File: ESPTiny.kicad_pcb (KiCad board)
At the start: 2 copper layers, 33 x 26.4 mm, 16 parts, among them J1 Conn_01x10_Male, J2 Conn_01x10_Male, J3 Conn_01x04_Male, U1 ESP-01v090, U2 ATtiny84-20PU, U3 MCP1700-3302E_TO92

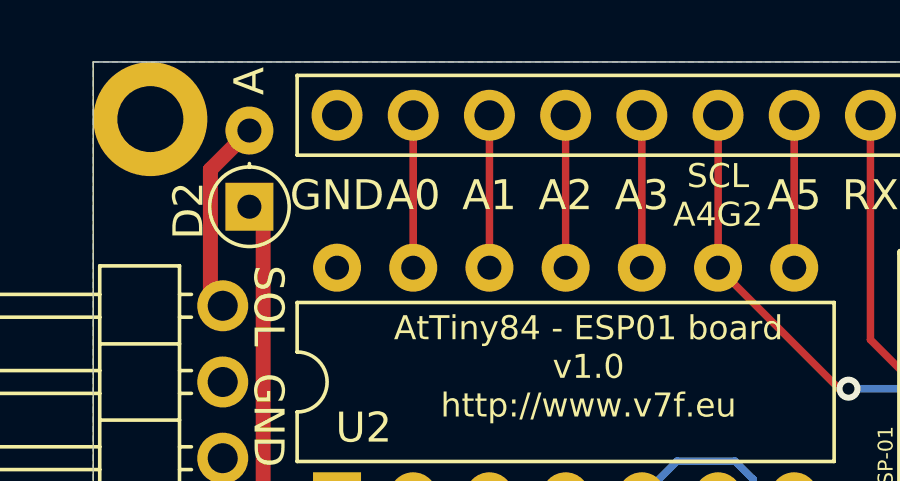
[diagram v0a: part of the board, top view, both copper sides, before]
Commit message: With power divider
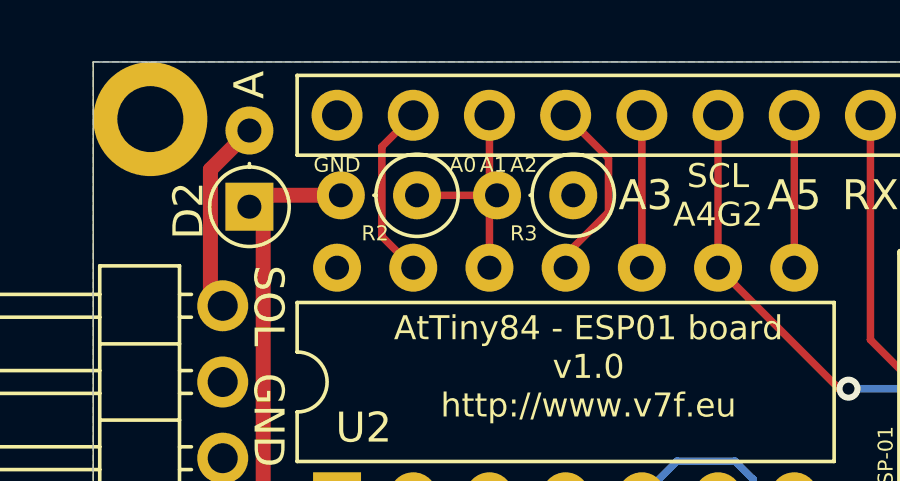
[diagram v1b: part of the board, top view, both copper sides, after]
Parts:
- added R2: 220, Resistor_THT:R_Axial_DIN0207_L6.3mm_D2.5mm_P2.54mm_Vertical, F.Cu at (49.9, 44.8)
- added R3: 220, Resistor_THT:R_Axial_DIN0207_L6.3mm_D2.5mm_P2.54mm_Vertical, F.Cu at (55.1, 44.8)
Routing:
- net +BATT: track 21.2 -> 24.4 mm
- net /A1: track 5.08 -> 7.96 mm
- net /A2: track 5.08 -> 6.26 mm
- net /A0: track 5.08 -> 5.95 mm
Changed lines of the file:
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@@
     (thickness 1.6)
     (drawings 49)
-    (tracks 122)
+    (tracks 133)
     (zones 0)
-    (modules 16)
+    (modules 18)
     (nets 21)
   )
@@
   )
   (layers
-    (0 F.Cu signal hide)
-    (31 B.Cu signal hide)
+    (0 F.Cu signal)
+    (31 B.Cu signal)
     (32 B.Adhes user)
     (33 F.Adhes user)
@@
       (effects (font (size 1 1) (thickness 0.15)))
     )
-    (fp_text user A (at 4.191 0 90) (layer F.SilkS)
+    (fp_text user A (at 4.064 0 90) (layer F.SilkS)
       (effects (font (size 1 1) (thickness 0.15)))
     )
@@
     )
   )
+  (module Resistor_THT:R_Axial_DIN0207_L6.3mm_D2.5mm_P2.54mm_Vertical (layer F.Cu)
+    (at 49.911 44.831 180)
+    (descr "Resistor, Axial_DIN0207 series, Axial, Vertical, pin pitch=2.54mm, 0.25W = 1/4W, length*diameter=6.3*2.5mm^2, http://cdn-reichelt.de/documents/datenblatt/B400/1_4W%23YAG.pdf")
+    (tags "Resistor Axial_DIN0207 series Axial Vertical pin pitch 2.54mm 0.25W = 1/4W length 6.3mm diameter 2.5mm")
+    (fp_text reference R2 (at 1.397 -1.27) (layer F.SilkS)
+      (effects (font (size 0.5 0.5) (thickness 0.125)))
+    )
+    (fp_text value 220 (at 1.27 2.37) (layer F.Fab)
+      (effects (font (size 1 1) (thickness 0.15)))
+    )
+    (fp_line (start 3.59 -1.5) (end -1.5 -1.5) (layer F.CrtYd) (width 0.05))
+    (fp_line (start 3.59 1.5) (end 3.59 -1.5) (layer F.CrtYd) (width 0.05))
+    (fp_line (start -1.5 1.5) (end 3.59 1.5) (layer F.CrtYd) (width 0.05))
+    (fp_line (start -1.5 -1.5) (end -1.5 1.5) (layer F.CrtYd) (width 0.05))
+    (fp_line (start 1.37 0) (end 1.44 0) (layer F.SilkS) (width 0.12))
+    (fp_line (start 0 0) (end 2.54 0) (layer F.Fab) (width 0.1))
+    (fp_circle (center 0 0) (end 1.37 0) (layer F.SilkS) (width 0.12))
+    (fp_circle (center 0 0) (end 1.25 0) (layer F.Fab) (width 0.1))
+    (fp_text user %R (at 1.27 -2.37) (layer F.Fab)
+      (effects (font (size 1 1) (thickness 0.15)))
+    )
+    (pad 1 thru_hole circle (at 0 0 180) (size 1.6 1.6) (drill 0.8) (layers *.Cu *.Mask)
+      (net 19 /A1))
+    (pad 2 thru_hole oval (at 2.54 0 180) (size 1.6 1.6) (drill 0.8) (layers *.Cu *.Mask)
+      (net 5 +BATT))
+    (model ${KISYS3DMOD}/Resistor_THT.3dshapes/R_Axial_DIN0207_L6.3mm_D2.5mm_P2.54mm_Vertical.wrl
+      (at (xyz 0 0 0))
+      (scale (xyz 1 1 1))
+      (rotate (xyz 0 0 0))
+    )
+  )
+  (module Resistor_THT:R_Axial_DIN0207_L6.3mm_D2.5mm_P2.54mm_Vertical (layer F.Cu)
+    (at 55.118 44.831 180)
+    (descr "Resistor, Axial_DIN0207 series, Axial, Vertical, pin pitch=2.54mm, 0.25W = 1/4W, length*diameter=6.3*2.5mm^2, http://cdn-reichelt.de/documents/datenblatt/B400/1_4W%23YAG.pdf")
+    (tags "Resistor Axial_DIN0207 series Axial Vertical pin pitch 2.54mm 0.25W = 1/4W length 6.3mm diameter 2.5mm")
+    (fp_text reference R3 (at 1.651 -1.27) (layer F.SilkS)
+      (effects (font (size 0.5 0.5) (thickness 0.125)))
+    )
+    (fp_text value 220 (at 1.27 2.37) (layer F.Fab)
+      (effects (font (size 1 1) (thickness 0.15)))
+    )
+    (fp_text user %R (at 1.27 -2.37) (layer F.Fab)
+      (effects (font (size 1 1) (thickness 0.15)))
+    )
+    (fp_circle (center 0 0) (end 1.25 0) (layer F.Fab) (width 0.1))
+    (fp_circle (center 0 0) (end 1.37 0) (layer F.SilkS) (width 0.12))
+    (fp_line (start 0 0) (end 2.54 0) (layer F.Fab) (width 0.1))
+    (fp_line (start 1.37 0) (end 1.44 0) (layer F.SilkS) (width 0.12))
+    (fp_line (start -1.5 -1.5) (end -1.5 1.5) (layer F.CrtYd) (width 0.05))
+    (fp_line (start -1.5 1.5) (end 3.59 1.5) (layer F.CrtYd) (width 0.05))
+    (fp_line (start 3.59 1.5) (end 3.59 -1.5) (layer F.CrtYd) (width 0.05))
+    (fp_line (start 3.59 -1.5) (end -1.5 -1.5) (layer F.CrtYd) (width 0.05))
+    (pad 2 thru_hole oval (at 2.54 0 180) (size 1.6 1.6) (drill 0.8) (layers *.Cu *.Mask)
+      (net 19 /A1))
+    (pad 1 thru_hole circle (at 0 0 180) (size 1.6 1.6) (drill 0.8) (layers *.Cu *.Mask)
+      (net 1 GND))
+    (model ${KISYS3DMOD}/Resistor_THT.3dshapes/R_Axial_DIN0207_L6.3mm_D2.5mm_P2.54mm_Vertical.wrl
+      (at (xyz 0 0 0))
+      (scale (xyz 1 1 1))
+      (rotate (xyz 0 0 0))
+    )
+  )
   (gr_text GND (at 71.374 43.053 270) (layer B.SilkS)
     (effects (font (size 0.5 0.5) (thickness 0.125)) (justify mirror))
@@
     (effects (font (size 1 1) (thickness 0.15)) (justify mirror))
   )
-  (gr_text A2 (at 54.864 44.831) (layer B.SilkS)
-    (effects (font (size 1 1) (thickness 0.15)) (justify mirror))
-  )
-  (gr_text A1 (at 52.197 44.831) (layer B.SilkS)
-    (effects (font (size 1 1) (thickness 0.15)) (justify mirror))
-  )
-  (gr_text A0 (at 49.784 44.831) (layer B.SilkS)
-    (effects (font (size 1 1) (thickness 0.15)) (justify mirror))
-  )
-  (gr_text GND (at 47.244 44.831) (layer B.SilkS)
-    (effects (font (size 1 1) (thickness 0.15)) (justify mirror))
+  (gr_text A2 (at 54.864 43.434) (layer B.SilkS)
+    (effects (font (size 0.5 0.5) (thickness 0.125)) (justify mirror))
+  )
+  (gr_text A1 (at 52.197 43.434) (layer B.SilkS)
+    (effects (font (size 0.5 0.5) (thickness 0.125)) (justify mirror))
+  )
+  (gr_text A0 (at 49.784 43.434) (layer B.SilkS)
+    (effects (font (size 0.5 0.5) (thickness 0.125)) (justify mirror))
+  )
+  (gr_text GND (at 47.244 43.434) (layer B.SilkS)
+    (effects (font (size 0.5 0.5) (thickness 0.125)) (justify mirror))
   )
   (gr_text 3V3 (at 70.612 65.913) (layer F.SilkS)
@@
     (effects (font (size 0.8 0.8) (thickness 0.15)))
   )
-  (gr_text A3 (at 57.404 44.831) (layer F.SilkS)
-    (effects (font (size 1 1) (thickness 0.15)))
-  )
-  (gr_text A2 (at 54.864 44.831) (layer F.SilkS)
-    (effects (font (size 1 1) (thickness 0.15)))
-  )
-  (gr_text A1 (at 52.324 44.831) (layer F.SilkS)
-    (effects (font (size 1 1) (thickness 0.15)))
-  )
-  (gr_text A0 (at 49.784 44.831) (layer F.SilkS)
-    (effects (font (size 1 1) (thickness 0.15)))
-  )
-  (gr_text GND (at 47.244 44.831) (layer F.SilkS)
-    (effects (font (size 1 1) (thickness 0.15)))
+  (gr_text A3 (at 57.531 44.831) (layer F.SilkS)
+    (effects (font (size 1 1) (thickness 0.15)))
+  )
+  (gr_text A2 (at 53.467 43.815) (layer F.SilkS)
+    (effects (font (size 0.5 0.5) (thickness 0.125)))
+  )
+  (gr_text A1 (at 52.451 43.815) (layer F.SilkS)
+    (effects (font (size 0.5 0.5) (thickness 0.125)))
+  )
+  (gr_text A0 (at 51.435 43.815) (layer F.SilkS)
+    (effects (font (size 0.5 0.5) (thickness 0.125)))
+  )
+  (gr_text GND (at 47.244 43.815) (layer F.SilkS)
+    (effects (font (size 0.5 0.5) (thickness 0.125)))
   )
   (gr_line (start 72.136 40.386) (end 72.136 66.802) (layer Edge.Cuts) (width 0.05))
@@
   (segment (start 44.784001 54.783999) (end 44.784001 45.673001) (width 0.5) (layer F.Cu) (net 5))
   (segment (start 43.434 56.134) (end 44.784001 54.783999) (width 0.5) (layer F.Cu) (net 5))
+  (segment (start 44.704 44.831) (end 44.323 45.212) (width 0.5) (layer F.Cu) (net 5))
+  (segment (start 47.371 44.831) (end 44.704 44.831) (width 0.5) (layer F.Cu) (net 5))
   (segment (start 51.721001 64.421001) (end 52.324 65.024) (width 0.25) (layer B.Cu) (net 6))
   (segment (start 51.943998 64.643998) (end 52.324 65.024) (width 0.25) (layer F.Cu) (net 6))
@@
   (segment (start 69.056601 51.276601) (end 64.293399 51.276601) (width 0.25) (layer B.Cu) (net 16))
   (segment (start 57.404 42.164) (end 57.404 47.244) (width 0.25) (layer F.Cu) (net 17))
-  (segment (start 54.864 42.164) (end 54.864 47.244) (width 0.25) (layer F.Cu) (net 18))
-  (segment (start 52.324 42.164) (end 52.324 47.244) (width 0.25) (layer F.Cu) (net 19))
-  (segment (start 49.784 47.244) (end 49.784 42.164) (width 0.25) (layer F.Cu) (net 20))
+  (segment (start 56.293001 43.593001) (end 54.864 42.164) (width 0.25) (layer F.Cu) (net 18))
+  (segment (start 56.293001 45.395001) (end 56.293001 43.593001) (width 0.25) (layer F.Cu) (net 18))
+  (segment (start 54.864 46.824002) (end 56.293001 45.395001) (width 0.25) (layer F.Cu) (net 18))
+  (segment (start 54.864 47.244) (end 54.864 46.824002) (width 0.25) (layer F.Cu) (net 18))
+  (segment (start 52.324 44.577) (end 52.578 44.831) (width 0.25) (layer F.Cu) (net 19))
+  (segment (start 52.324 42.164) (end 52.324 44.577) (width 0.25) (layer F.Cu) (net 19))
+  (segment (start 52.324 45.085) (end 52.578 44.831) (width 0.25) (layer F.Cu) (net 19))
+  (segment (start 52.324 47.244) (end 52.324 45.085) (width 0.25) (layer F.Cu) (net 19))
+  (segment (start 52.578 44.831) (end 49.911 44.831) (width 0.25) (layer F.Cu) (net 19))
+  (segment (start 48.735999 43.212001) (end 49.784 42.164) (width 0.25) (layer F.Cu) (net 20))
+  (segment (start 48.735999 46.195999) (end 48.735999 43.212001) (width 0.25) (layer F.Cu) (net 20))
+  (segment (start 49.784 47.244) (end 48.735999 46.195999) (width 0.25) (layer F.Cu) (net 20))
   (zone (net 1) (net_name GND) (layer B.Cu) (hatch edge 0.508)
     (connect_pads (clearance 0.508))
